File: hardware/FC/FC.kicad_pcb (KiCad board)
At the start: 2 copper layers, 52 parts, among them CN1 HC-0.8-8PWT, J1 USB-C, SW1 TS-1088-AR02016, SW2 TS-1088-AR02016, U1 STM32F722RET6, U2 TPS63070RNMR, U4 ICM-20602, U5 AP2112K-3.3TRG1, U6 BMP580, X1 X322525MOB4SI, X2 Q13FC1350000400

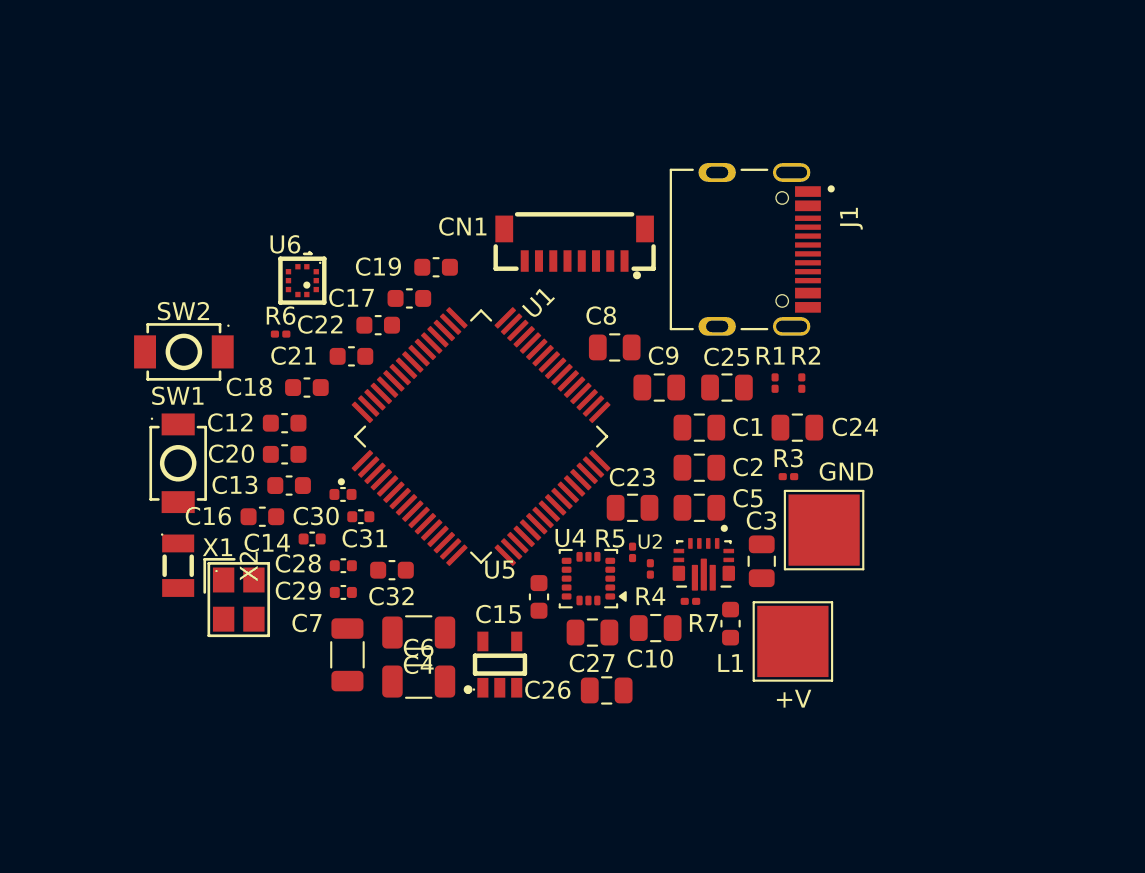
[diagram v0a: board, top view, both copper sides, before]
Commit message: added pcb design
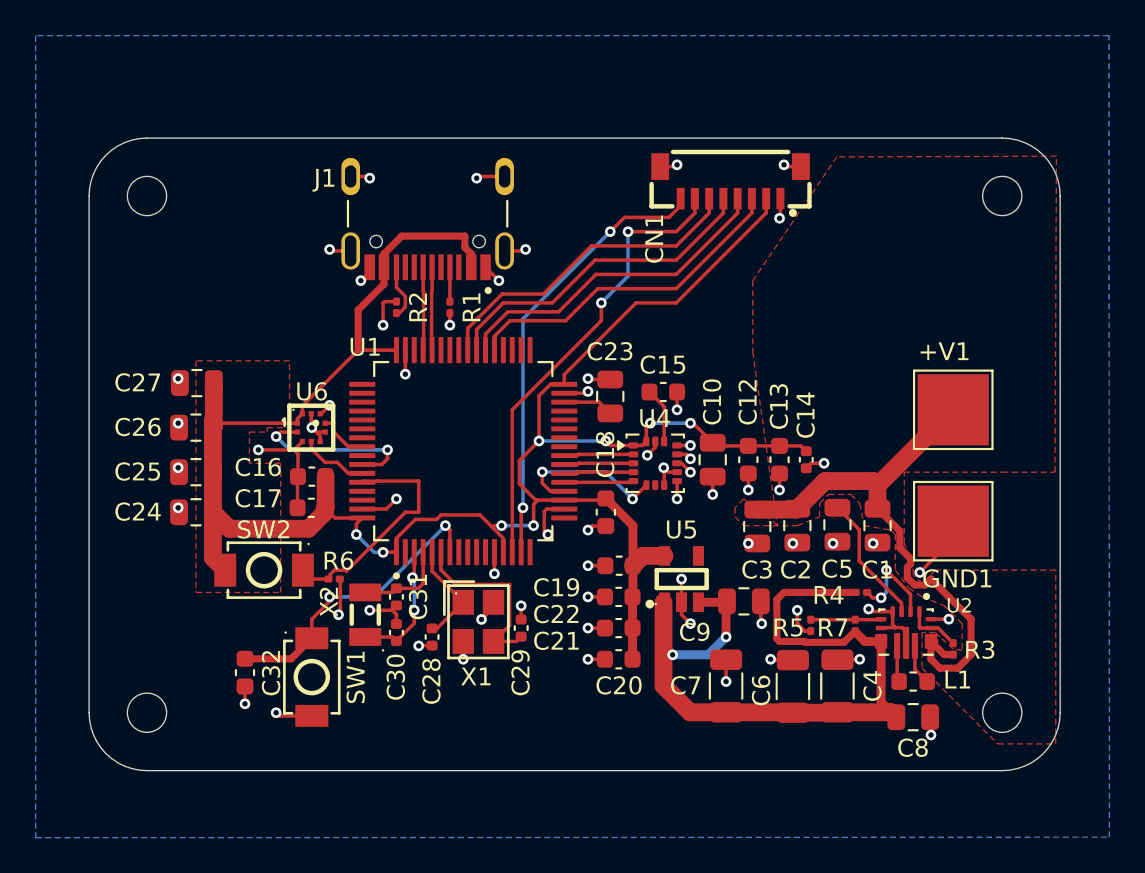
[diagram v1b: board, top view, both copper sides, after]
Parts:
- added H1: MountingHole, MountingHole:MountingHole_2.2mm_M2, F.Cu at (131.2, 115.5)
- added H2: MountingHole, MountingHole:MountingHole_2.2mm_M2, F.Cu at (131.2, 86.5)
- added H3: MountingHole, MountingHole:MountingHole_2.2mm_M2, F.Cu at (179.2, 86.5)
- added H4: MountingHole, MountingHole:MountingHole_2.2mm_M2, F.Cu at (179.2, 115.5)
- moved C24 34.1 mm to (134.0, 104.2), turned to 180 degrees
- moved C25 30.2 mm to (134.0, 102.0), turned to 180 degrees
- moved C14 28.1 mm to (168.2, 101.3), turned to -90 degrees
- moved C13 27.6 mm to (166.8, 101.3), turned to 90 degrees
- moved C26 27.4 mm to (134.0, 99.5)
- moved C8 26.7 mm to (174.2, 115.8), turned to 0 degrees
- moved C27 26.2 mm to (134.1, 97.0)
- moved C12 26.1 mm to (165.0, 101.3), turned to 90 degrees
- moved C4 23.7 mm to (170.0, 114.0), turned to 90 degrees
- moved R2 23.1 mm to (145.2, 92.8)
- moved C20 22.0 mm to (157.7, 112.5), turned to 180 degrees
- moved C21 21.4 mm to (157.7, 110.8), turned to 180 degrees
- moved C7 21.3 mm to (163.8, 114.0)
- moved C6 21.0 mm to (167.5, 114.0), turned to 90 degrees
- moved C22 20.4 mm to (157.7, 109.0), turned to 180 degrees
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- renumbered +V to +V1, GND to GND1
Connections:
- C28 pad 2: Net-(X1-OSC1) -> /HSE_IN
- C29 pad 1: Net-(X1-OSC2) -> GND
- C29 pad 2: GND -> /HSE_OUT
- J1 pad A4B9: VBUS -> +3V3
- J1 pad A8: /SBU1 -> unconnected-(J1-SBU1-PadA8)
- J1 pad B4A9: VBUS -> +3V3
- J1 pad B8: /SBU2 -> unconnected-(J1-SBU2-PadB8)
- U1 pad 15: unconnected-(U1-PA1-Pad15) -> /ESC_TELE
- U1 pad 20: /ICM_CS -> /ICM_INT
- U1 pad 21: /ICM_SCK -> /ICM_CS
- U1 pad 24: unconnected-(U1-PC4-Pad24) -> /ICM_SCK
- U1 pad 44: /USB_D1- -> /USB_D1+
- U1 pad 45: /USB_D1+ -> /USB_D1-
- U1 pad 5: GND -> /HSE_IN
- U1 pad 51: /ESC_TELE -> unconnected-(U1-PC10-Pad51)
- U1 pad 6: GND -> /HSE_OUT
- X1 pad 1: Net-(X1-OSC1) -> /HSE_IN
- X1 pad 3: Net-(X1-OSC2) -> /HSE_OUT
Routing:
- net +3V3: track 0.00 -> 121.0 mm, vias 0 -> 8
- net GND: track 0.00 -> 81.9 mm, vias 0 -> 63
- net +5V: track 0.00 -> 46.0 mm, vias 0 -> 2
- net /VSYS: track 0.00 -> 31.9 mm
- net /ESC_CURR: track 0.00 -> 25.7 mm, vias 0 -> 2
- net /ESC_TELE: track 0.00 -> 25.0 mm, vias 0 -> 2
- net /ESC1: track 0.00 -> 18.9 mm
- net /ESC2: track 0.00 -> 18.7 mm
- net /ESC3: track 0.00 -> 18.5 mm
- net /ESC4: track 0.00 -> 18.3 mm
- net /RESET: track 0.00 -> 16.7 mm, vias 0 -> 2
- net /BOOT: track 0.00 -> 13.4 mm
- net /HSE_OUT: track 0.00 -> 10.4 mm
- net /I2C_SCL: track 0.00 -> 9.91 mm, vias 0 -> 2
- net /ICM_INT: track 0.00 -> 8.84 mm, vias 0 -> 2
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- added copper zone on F.Cu, net +3V3
- added copper zone on F.Cu, net /VSYS
- added copper zone on B.Cu, net GND
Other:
- board outline added: 54.5 x 35.5 mm
